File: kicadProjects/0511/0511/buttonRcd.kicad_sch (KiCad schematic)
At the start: 5 parts, among them SW1 SW_Push

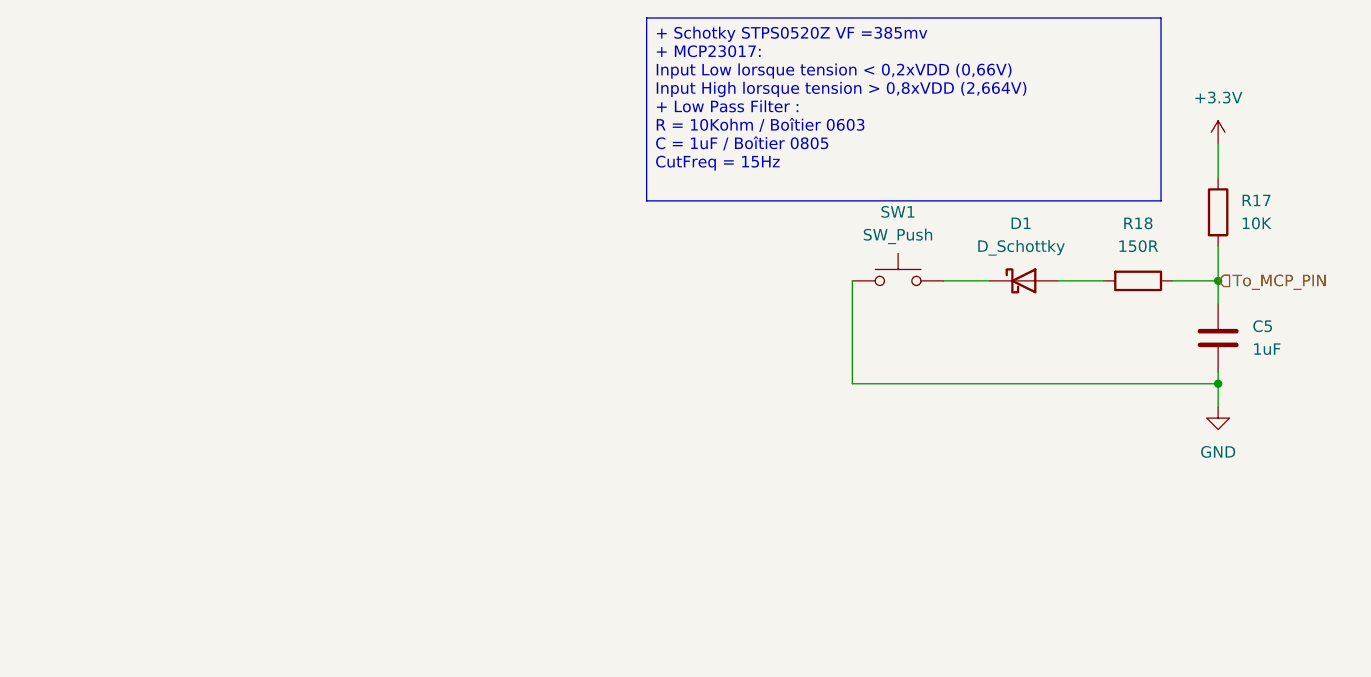
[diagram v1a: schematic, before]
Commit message: assignation empreintes
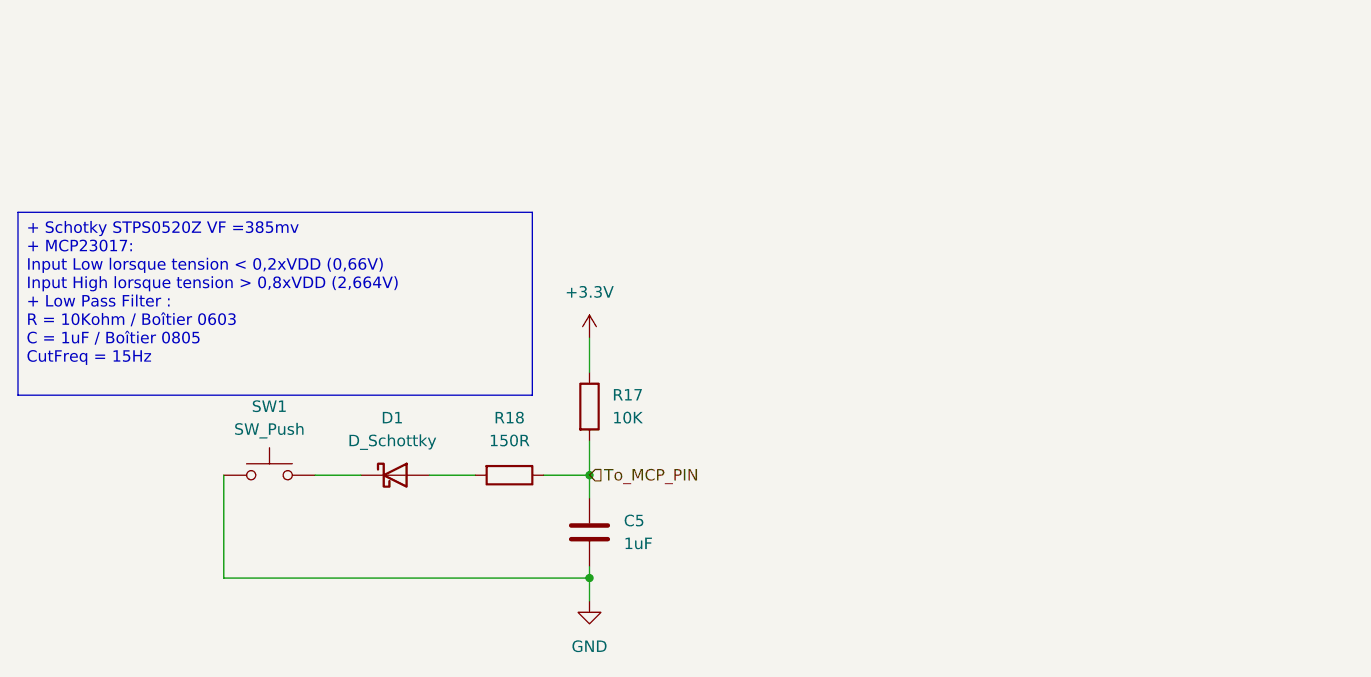
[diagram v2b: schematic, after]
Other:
- moved on the sheet: C5, D1, R17, R18, SW1
